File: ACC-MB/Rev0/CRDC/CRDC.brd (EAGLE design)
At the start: 84 x 61.5 mm, 5 parts

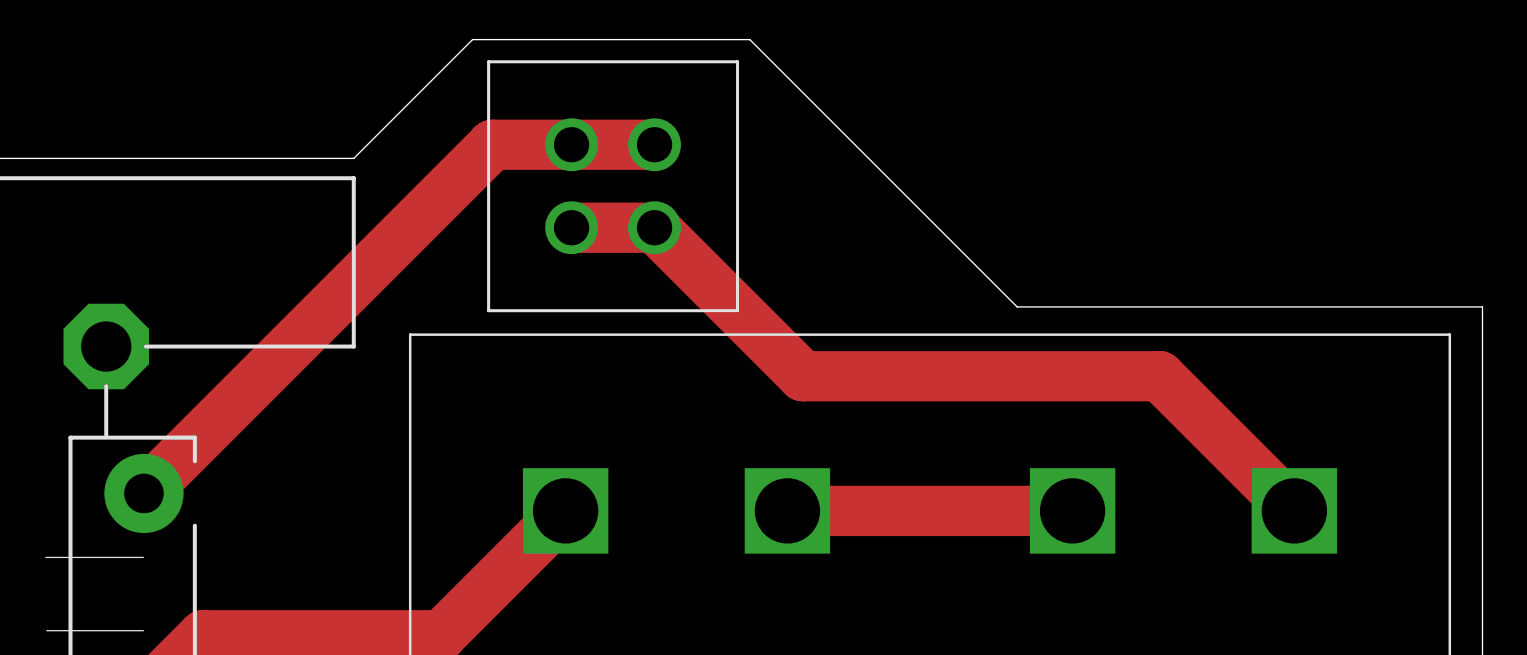
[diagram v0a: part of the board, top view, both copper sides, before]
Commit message: update
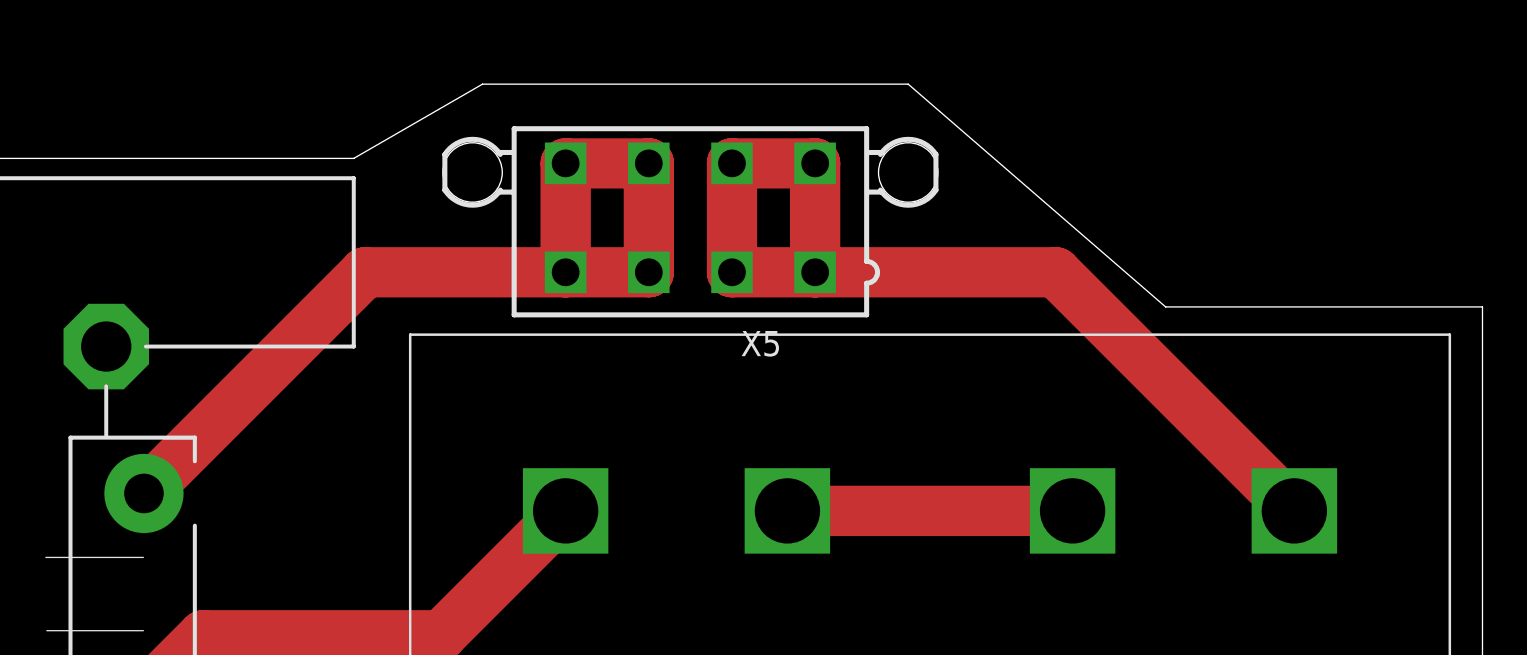
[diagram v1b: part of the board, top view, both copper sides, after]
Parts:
- removed U$4: IPBT-102-H1-T-D, ACC-MB-R0:IPBT-102-H1-T-D
- added X5: 5566-8, con-molex:5566-8
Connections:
- net HV+_WET: now also X5.3, X5.4, X5.7, X5.8; no longer U$4.P$3, U$4.P$4
- net V+: now also X5.1, X5.2, X5.5, X5.6; no longer U$4.P$1, U$4.P$2
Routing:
- net HV+_WET: track 33.1 -> 45.3 mm
- net V+: track 41.9 -> 48.6 mm
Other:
- board size 84 x 61.5 mm -> 84 x 59.2 mm
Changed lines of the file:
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@@
 <drawing>
 <settings>
-<setting alwaysvectorfont="yes"/>
+<setting alwaysvectorfont="no"/>
 <setting verticaltext="up"/>
 </settings>
@@
 <wire x1="20" y1="9.5" x2="30.5" y2="9.5" width="0" layer="20"/>
 <wire x1="55.5" y1="9.5" x2="64" y2="9.5" width="0" layer="20"/>
-<wire x1="84" y1="46" x2="60.5" y2="46" width="0" layer="20"/>
-<wire x1="60.5" y1="46" x2="47" y2="59.5" width="0" layer="20"/>
-<wire x1="47" y1="59.5" x2="33" y2="59.5" width="0" layer="20"/>
-<wire x1="33" y1="59.5" x2="27" y2="53.5" width="0" layer="20"/>
+<wire x1="84" y1="46" x2="68" y2="46" width="0" layer="20"/>
+<wire x1="68" y1="46" x2="55" y2="57.25" width="0" layer="20"/>
+<wire x1="55" y1="57.25" x2="33.5" y2="57.25" width="0" layer="20"/>
+<wire x1="33.5" y1="57.25" x2="27" y2="53.5" width="0" layer="20"/>
 <wire x1="27" y1="53.5" x2="0" y2="53.5" width="0" layer="20"/>
 <wire x1="0" y1="9.5" x2="0" y2="-1.75" width="0" layer="20"/>
@@
 <elements>
 <element name="U$1" library="ACC-MB-R0" library_urn="urn:adsk.eagle:library:13324935" package="G7L" package3d_urn="urn:adsk.eagle:package:13209535/2" value="G7L" x="74.5" y="18" rot="R180"/>
-<element name="U$4" library="ACC-MB-R0" library_urn="urn:adsk.eagle:library:13324935" package="IPBT-102-H1-T-D" package3d_urn="urn:adsk.eagle:package:13324986/2" value="IPBT-102-H1-T-D" x="38" y="50"/>
 <element name="U$5" library="ACC-MB-R0" library_urn="urn:adsk.eagle:library:13324935" package="_CUSTOM_TO-247-2V" package3d_urn="urn:adsk.eagle:package:13209502/3" value="TO247RESISTORHEATINK" x="14.5" y="31.5" rot="R90">
 <attribute name="MPN" value="" x="14.5" y="31.5" size="1.778" layer="27" rot="R90" display="off"/>
@@
 <element name="U$2" library="ACC-MB-R0" library_urn="urn:adsk.eagle:library:13324935" package="PCI-E_SLOT_36" value="PCIE-36-EDGE" x="64.25" y="-2"/>
 <element name="U$3" library="ACC-MB-R0" library_urn="urn:adsk.eagle:library:13324935" package="PCI-E_SLOT_36" value="PCIE-36-EDGE" x="0.25" y="-2"/>
+<element name="X5" library="con-molex" library_urn="urn:adsk.eagle:library:165" package="5566-8" value="5566-8" x="44" y="50.5">
+<attribute name="MF" value="MOLEX" x="44" y="50.5" size="1.778" layer="27" display="off"/>
+<attribute name="MPN" value="" x="44" y="50.5" size="1.778" layer="27" display="off"/>
+<attribute name="OC_FARNELL" value="unknown" x="44" y="50.5" size="1.778" layer="27" display="off"/>
+<attribute name="OC_NEWARK" value="unknown" x="44" y="50.5" size="1.778" layer="27" display="off"/>
+</element>
 </elements>
 <signals>
 <signal name="HV+_WET">
-<contactref element="U$4" pad="P$3"/>
-<contactref element="U$4" pad="P$4"/>
-<wire x1="42.19" y1="54.19" x2="38" y2="54.19" width="2.54" layer="1"/>
 <contactref element="U$5" pad="2"/>
-<wire x1="16.405" y1="36.58" x2="34.015" y2="54.19" width="2.54" layer="1"/>
-<wire x1="34.015" y1="54.19" x2="38" y2="54.19" width="2.54" layer="1"/>
+<contactref element="X5" pad="4"/>
+<contactref element="X5" pad="3"/>
+<wire x1="16.405" y1="36.58" x2="27.575" y2="47.75" width="2.54" layer="1"/>
+<wire x1="27.575" y1="47.75" x2="37.7" y2="47.75" width="2.54" layer="1"/>
+<contactref element="X5" pad="7"/>
+<contactref element="X5" pad="8"/>
+<wire x1="37.7" y1="47.75" x2="41.9" y2="47.75" width="2.54" layer="1"/>
+<wire x1="41.9" y1="47.75" x2="41.9" y2="53.25" width="2.54" layer="1"/>
+<wire x1="41.9" y1="53.25" x2="37.7" y2="53.25" width="2.54" layer="1"/>
+<wire x1="37.7" y1="53.25" x2="37.7" y2="47.75" width="2.54" layer="1"/>
 </signal>
 <signal name="N$21">
@@
 <signal name="V+" class="1">
 <contactref element="U$1" pad="2"/>
-<contactref element="U$4" pad="P$1"/>
-<contactref element="U$4" pad="P$2"/>
-<wire x1="74.5" y1="35.7" x2="67.7" y2="42.5" width="2.54" layer="1"/>
-<wire x1="67.7" y1="42.5" x2="49.69" y2="42.5" width="2.54" layer="1"/>
-<wire x1="42.19" y1="50" x2="38.5" y2="50" width="2.54" layer="1"/>
-<wire x1="49.69" y1="42.5" x2="42.19" y2="50" width="2.54" layer="1"/>
-<wire x1="38" y1="50" x2="38.5" y2="50" width="0" layer="19" extent="1-1"/>
+<contactref element="X5" pad="5"/>
+<contactref element="X5" pad="6"/>
+<contactref element="X5" pad="2"/>
+<contactref element="X5" pad="1"/>
+<wire x1="50.3" y1="47.75" x2="62.45" y2="47.75" width="2.54" layer="1"/>
+<wire x1="62.45" y1="47.75" x2="74.5" y2="35.7" width="2.54" layer="1"/>
+<wire x1="50.3" y1="47.75" x2="46.1" y2="47.75" width="2.54" layer="1"/>
+<wire x1="46.1" y1="47.75" x2="46.1" y2="53.25" width="2.54" layer="1"/>
+<wire x1="46.1" y1="53.25" x2="50.3" y2="53.25" width="2.54" layer="1"/>
+<wire x1="50.3" y1="53.25" x2="50.3" y2="47.75" width="2.54" layer="1"/>
 </signal>
 <signal name="N$2">
